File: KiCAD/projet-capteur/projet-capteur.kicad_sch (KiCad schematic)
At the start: 21 parts, among them J1 Power, J2 Analog, J3 Digital/PWM, J4 Digital/PWM, U2 LTC1050

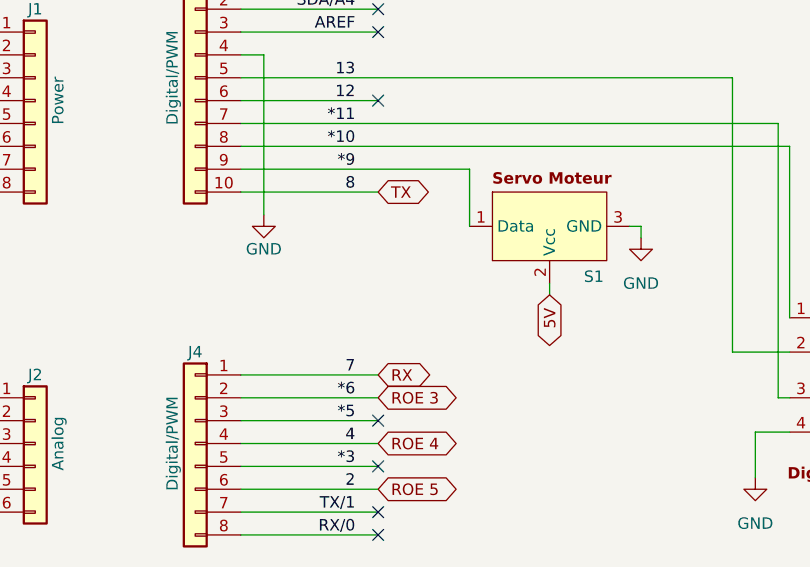
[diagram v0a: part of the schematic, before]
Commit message: Beautification du PCB
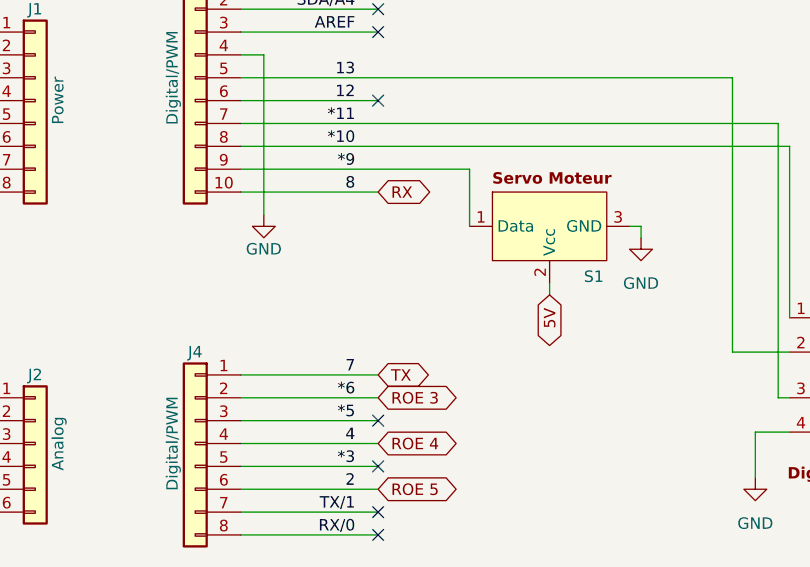
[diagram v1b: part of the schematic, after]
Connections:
- net RX: now also J3.10 (Pin_10); no longer J4.1 (Pin_1)
- net TX: now also J4.1 (Pin_1); no longer J3.10 (Pin_10)
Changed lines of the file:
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@@
 		)
 	)
-	(global_label "TX"
+	(global_label "ADC"
+		(shape bidirectional)
+		(at 34.29 68.58 180)
+		(fields_autoplaced yes)
+		(effects
+			(font
+				(size 1.27 1.27)
+			)
+			(justify right)
+		)
+		(property "Intersheetrefs" "${INTERSHEET_REFS}"
+			(at 26.5651 68.58 0)
+			(effects
+				(font
+					(size 1.27 1.27)
+				)
+				(justify right)
+				(hide yes)
+			)
+		)
+	)
+	(global_label "5V"
+		(shape bidirectional)
+		(at 101.6 62.23 270)
+		(fields_autoplaced yes)
+		(effects
+			(font
+				(size 1.27 1.27)
+			)
+			(justify right)
+		)
+		(property "Intersheetrefs" "${INTERSHEET_REFS}"
+			(at 101.6 68.6244 90)
+			(effects
+				(font
+					(size 1.27 1.27)
+				)
+				(justify right)
+				(hide yes)
+			)
+		)
+	)
+	(global_label "5V"
+		(shape bidirectional)
+		(at 104.14 102.87 180)
+		(fields_autoplaced yes)
+		(effects
+			(font
+				(size 1.27 1.27)
+			)
+			(justify right)
+		)
+		(property "Intersheetrefs" "${INTERSHEET_REFS}"
+			(at 97.7456 102.87 0)
+			(effects
+				(font
+					(size 1.27 1.27)
+				)
+				(justify right)
+				(hide yes)
+			)
+		)
+	)
+	(global_label "ADC"
+		(shape bidirectional)
+		(at 160.02 151.13 0)
+		(fields_autoplaced yes)
+		(effects
+			(font
+				(size 1.27 1.27)
+			)
+			(justify left)
+		)
+		(property "Intersheetrefs" "${INTERSHEET_REFS}"
+			(at 167.7449 151.13 0)
+			(effects
+				(font
+					(size 1.27 1.27)
+				)
+				(justify left)
+				(hide yes)
+			)
+		)
+	)
+	(global_label "RX"
 		(shape bidirectional)
 		(at 82.55 50.8 0)
@@
 		)
 		(property "Intersheetrefs" "${INTERSHEET_REFS}"
-			(at 88.8234 50.8 0)
-			(effects
-				(font
-					(size 1.27 1.27)
-				)
-				(justify left)
-				(hide yes)
-			)
-		)
-	)
-	(global_label "ADC"
-		(shape bidirectional)
-		(at 34.29 68.58 180)
-		(fields_autoplaced yes)
-		(effects
-			(font
-				(size 1.27 1.27)
-			)
-			(justify right)
-		)
-		(property "Intersheetrefs" "${INTERSHEET_REFS}"
-			(at 26.5651 68.58 0)
-			(effects
-				(font
-					(size 1.27 1.27)
-				)
-				(justify right)
-				(hide yes)
-			)
-		)
-	)
-	(global_label "5V"
-		(shape bidirectional)
-		(at 101.6 62.23 270)
-		(fields_autoplaced yes)
-		(effects
-			(font
-				(size 1.27 1.27)
-			)
-			(justify right)
-		)
-		(property "Intersheetrefs" "${INTERSHEET_REFS}"
-			(at 101.6 68.6244 90)
-			(effects
-				(font
-					(size 1.27 1.27)
-				)
-				(justify right)
-				(hide yes)
-			)
-		)
-	)
-	(global_label "5V"
-		(shape bidirectional)
-		(at 104.14 102.87 180)
-		(fields_autoplaced yes)
-		(effects
-			(font
-				(size 1.27 1.27)
-			)
-			(justify right)
-		)
-		(property "Intersheetrefs" "${INTERSHEET_REFS}"
-			(at 97.7456 102.87 0)
-			(effects
-				(font
-					(size 1.27 1.27)
-				)
-				(justify right)
-				(hide yes)
-			)
-		)
-	)
-	(global_label "ADC"
-		(shape bidirectional)
-		(at 160.02 151.13 0)
-		(fields_autoplaced yes)
-		(effects
-			(font
-				(size 1.27 1.27)
-			)
-			(justify left)
-		)
-		(property "Intersheetrefs" "${INTERSHEET_REFS}"
-			(at 167.7449 151.13 0)
+			(at 89.1258 50.8 0)
 			(effects
 				(font
@@
 		)
 	)
-	(global_label "RX"
+	(global_label "5V"
+		(shape bidirectional)
+		(at 152.4 64.77 0)
+		(fields_autoplaced yes)
+		(effects
+			(font
+				(size 1.27 1.27)
+			)
+			(justify left)
+		)
+		(property "Intersheetrefs" "${INTERSHEET_REFS}"
+			(at 158.7944 64.77 0)
+			(effects
+				(font
+					(size 1.27 1.27)
+				)
+				(justify left)
+				(hide yes)
+			)
+		)
+	)
+	(global_label "R3"
+		(shape bidirectional)
+		(at 152.4 68.58 0)
+		(fields_autoplaced yes)
+		(effects
+			(font
+				(size 1.27 1.27)
+			)
+			(justify left)
+		)
+		(property "Intersheetrefs" "${INTERSHEET_REFS}"
+			(at 158.9758 68.58 0)
+			(effects
+				(font
+					(size 1.27 1.27)
+				)
+				(justify left)
+				(hide yes)
+			)
+		)
+	)
+	(global_label "TX"
 		(shape bidirectional)
 		(at 82.55 71.12 0)
@@
 		)
 		(property "Intersheetrefs" "${INTERSHEET_REFS}"
-			(at 89.1258 71.12 0)
-			(effects
-				(font
-					(size 1.27 1.27)
-				)
-				(justify left)
-				(hide yes)
-			)
-		)
-	)
-	(global_label "5V"
-		(shape bidirectional)
-		(at 152.4 64.77 0)
-		(fields_autoplaced yes)
-		(effects
-			(font
-				(size 1.27 1.27)
-			)
-			(justify left)
-		)
-		(property "Intersheetrefs" "${INTERSHEET_REFS}"
-			(at 158.7944 64.77 0)
-			(effects
-				(font
-					(size 1.27 1.27)
-				)
-				(justify left)
-				(hide yes)
-			)
-		)
-	)
-	(global_label "R3"
-		(shape bidirectional)
-		(at 152.4 68.58 0)
-		(fields_autoplaced yes)
-		(effects
-			(font
-				(size 1.27 1.27)
-			)
-			(justify left)
-		)
-		(property "Intersheetrefs" "${INTERSHEET_REFS}"
-			(at 158.9758 68.58 0)
-			(effects
-				(font
+			(at 88.8234 71.12 0)
+			(effects
+				(font
